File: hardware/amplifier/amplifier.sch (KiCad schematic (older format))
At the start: 47 parts, among them IC3 AD8331, IC4 ISL55210, P1 OUT, P2 OUT, X1 IN

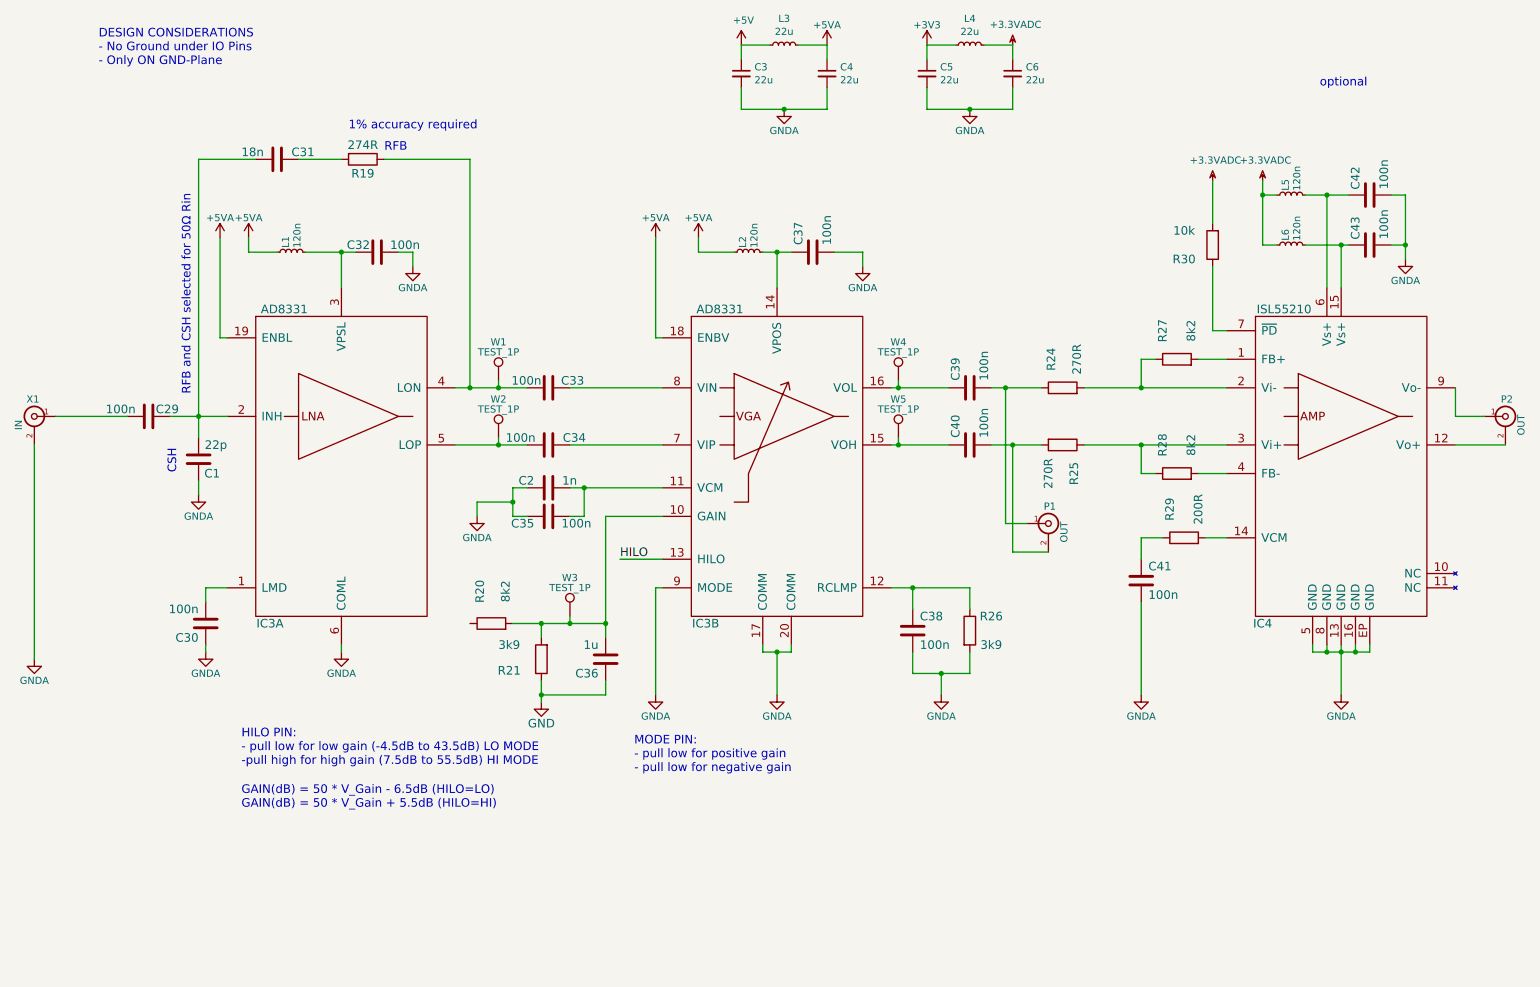
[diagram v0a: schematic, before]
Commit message: amp done
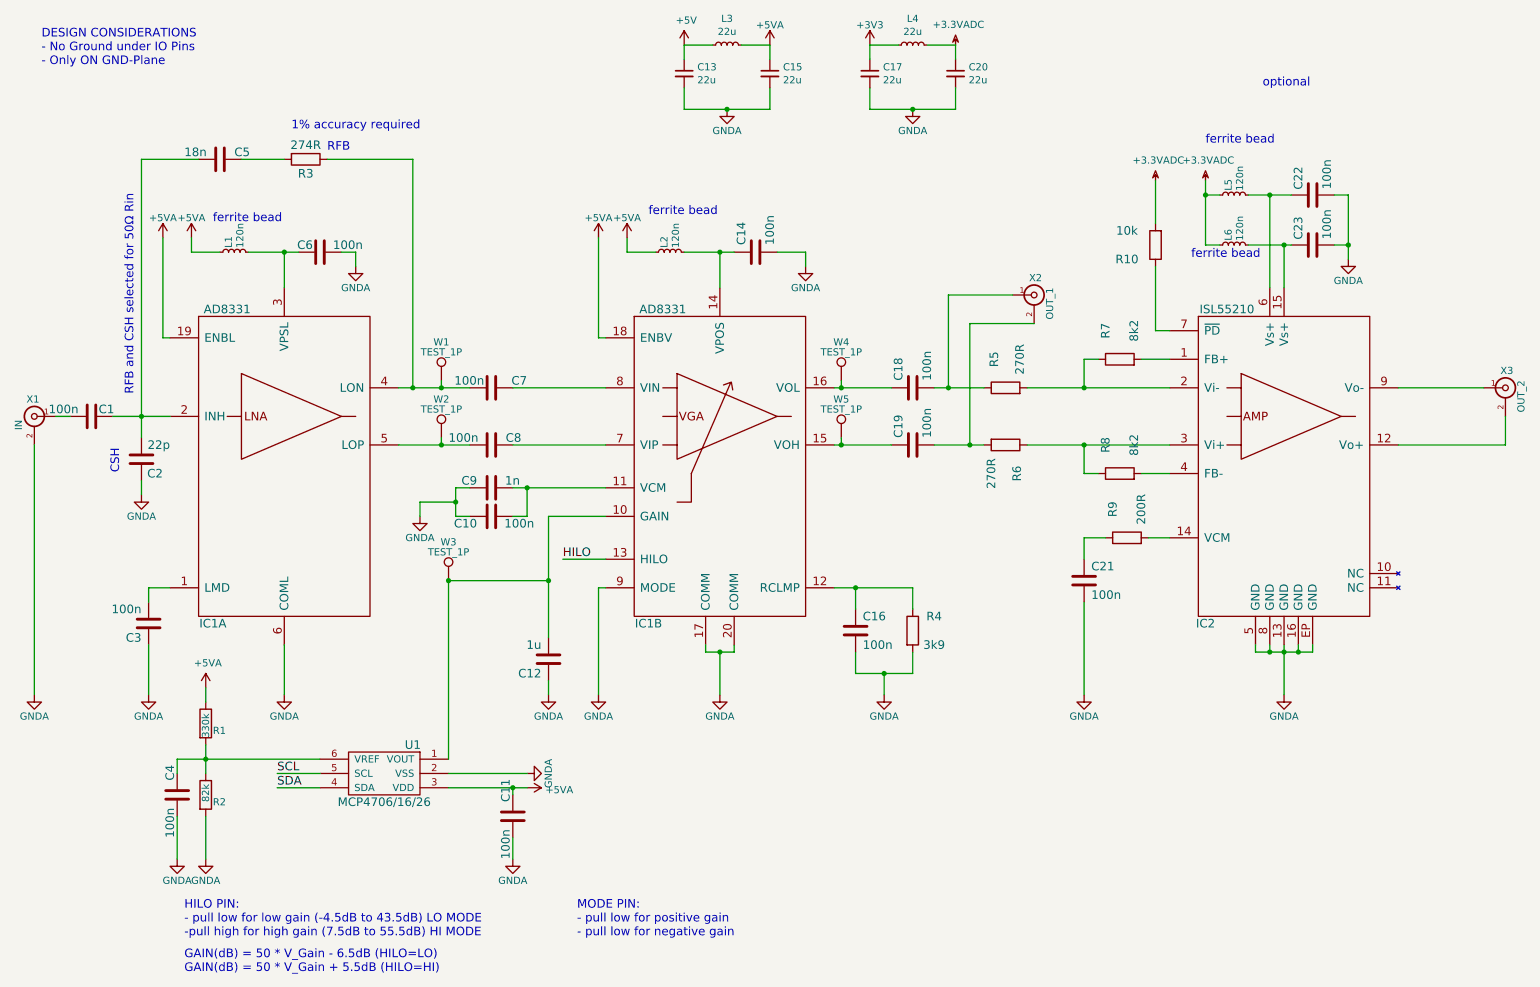
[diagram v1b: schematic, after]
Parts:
- removed R20: 8k2, Resistors_SMD:R_0603, symbol R
- removed R21: 3k9, Resistors_SMD:R_0603, symbol R
- added C11, C4: 100n, Capacitors_SMD:C_0603, symbol C
- added R1: 330k, Resistors_SMD:R_0603, symbol R
- added R2: 82k, Resistors_SMD:R_0603, symbol R
- added U1: MCP4706/16/26, TO_SOT_Packages_SMD:SOT-23-6, symbol MCP4706/16/26
- X2: renamed from P1; value OUT -> OUT_1
- X3: renamed from P2; value OUT -> OUT_2
- renumbered C29 to C1, C35 to C10, C36 to C12, C3 to C13, C37 to C14, C4 to C15, C38 to C16, C5 to C17, C39 to C18, C40 to C19, C1 to C2, C6 to C20, C41 to C21, C42 to C22, C43 to C23, C30 to C3, C31 to C5, C32 to C6, C33 to C7, C34 to C8, C2 to C9, IC3 to IC1, IC4 to IC2, R30 to R10, R19 to R3, R26 to R4, R24 to R5, R25 to R6, R27 to R7, R28 to R8, R29 to R9
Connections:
- net GND is gone; now on net GNDA: C12.1
- net +5VA: now also C11.1, R1.1, U1.3 (VDD)
- net GNDA: now also C11.2, C4.2, R2.2, U1.2 (VSS)
- net at C12.2, IC1.10 (GAIN), W3.1: now also U1.1 (VOUT)
- new net: C4.1, R1.2, R2.1, U1.6 (VREF)
- new net SCL: U1.5 (SCL)
- new net SDA: U1.4 (SDA)
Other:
- note added: "ferrite bead"
- moved on the sheet: C1, C10, C12, C13, C14, C15, C16, C17, C18, C19, C2, C20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
